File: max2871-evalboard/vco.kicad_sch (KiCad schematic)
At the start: 44 parts

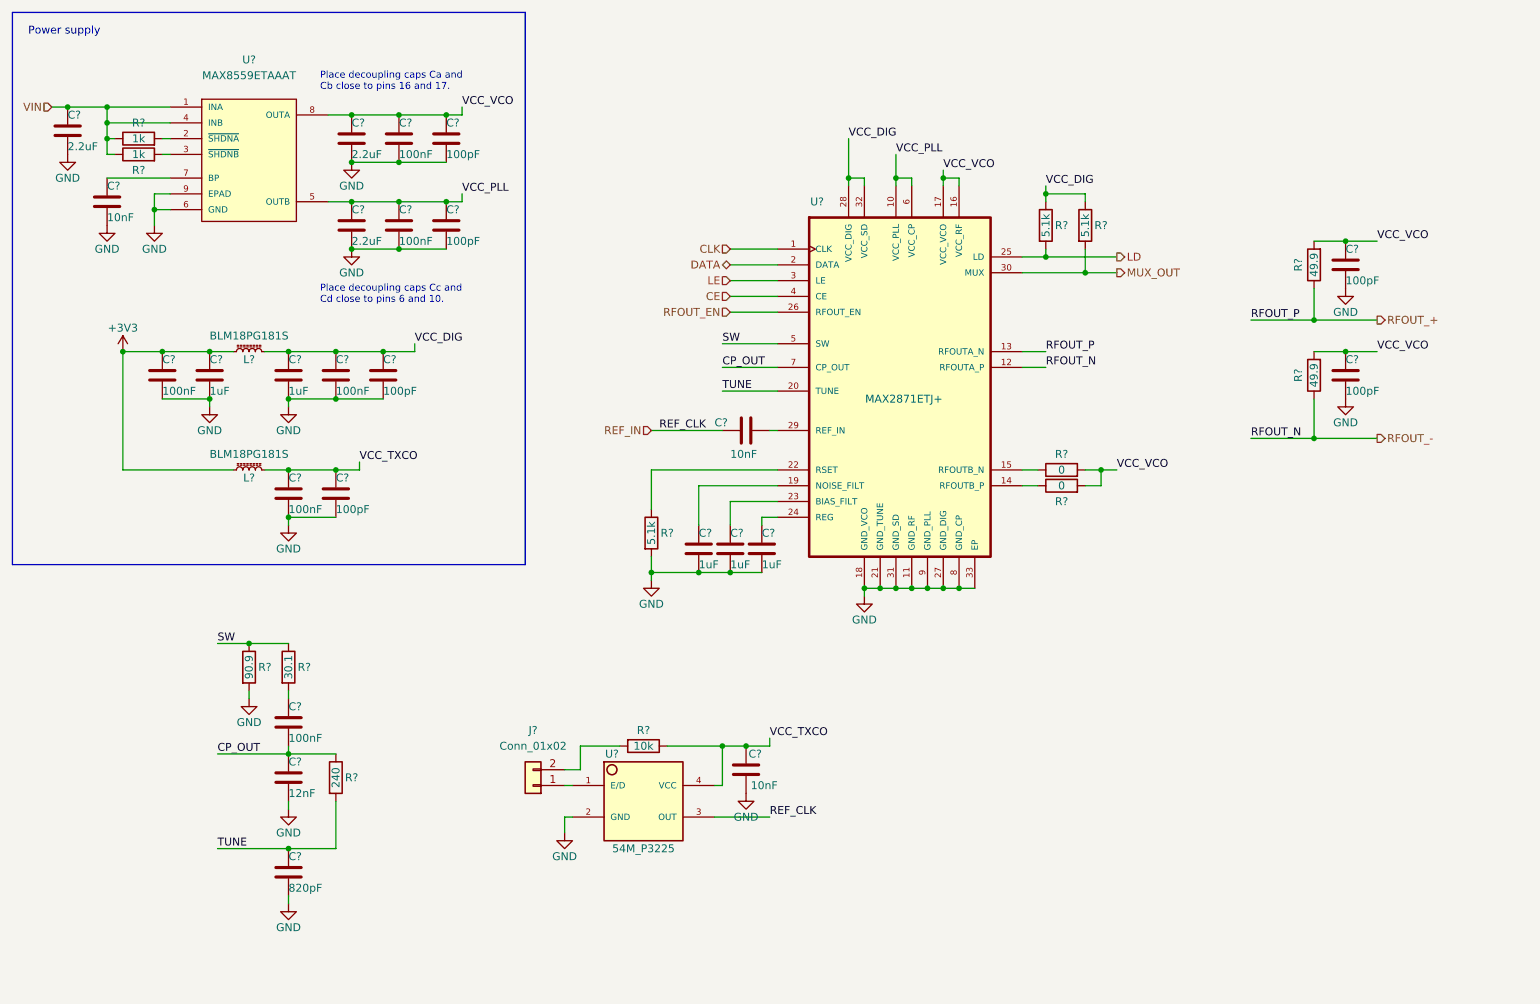
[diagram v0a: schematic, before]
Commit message: Finish schematic - create PCB
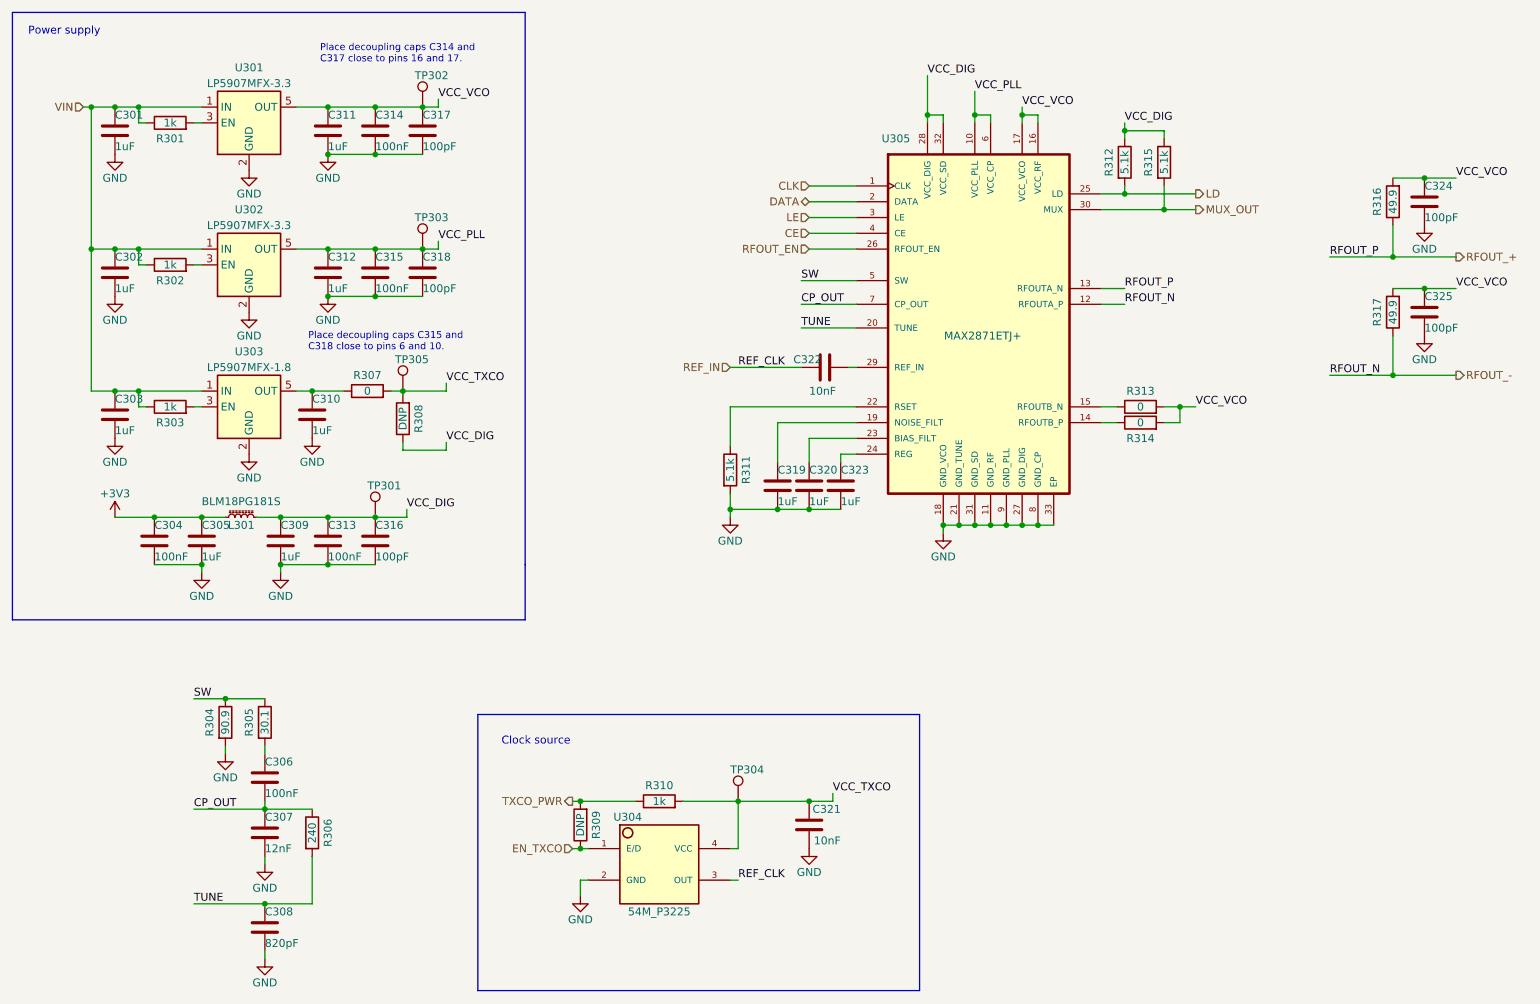
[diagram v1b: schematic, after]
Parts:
- removed C? (x3): 2.2uF, Capacitor_SMD:C_0603_1608Metric, symbol Device:C
- removed C?: 1uF, Capacitor_SMD:C_0402_1005Metric, symbol Device:C
- removed C?: 100pF, Capacitor_SMD:C_0402_1005Metric, symbol Device:C
- removed C?: 10nF, Capacitor_SMD:C_0402_1005Metric, symbol Device:C
- removed C?: 100nF, Capacitor_SMD:C_0402_1005Metric, symbol Device:C
- removed J?: Conn_01x02, Connector_PinHeader_2.54mm:PinHeader_2x01_P2.54mm_Horizontal, symbol Connector_Generic:Conn_01x02
- removed L?: BLM18PG181S, Inductor_SMD:L_0603_1608Metric, symbol Device:L_Ferrite_Small
- removed R?: 1k, Resistor_SMD:R_0402_1005Metric, symbol Device:R
- removed R?: 10k, Resistor_SMD:R_0402_1005Metric, symbol Device:R
- removed U?: MAX8559ETAAAT, MAX8559ETAAAT:SON65P300X300X80-9N, symbol MAX8559ETAAAT:MAX8559ETAAAT
- added C301, C302, C303, C309, C310, C311, C312: 1uF, Capacitor_SMD:C_0402_1005Metric, symbol Device:C
- added R301, R303, R310: 1k, Resistor_SMD:R_0402_1005Metric, symbol Device:R
- added R307: 0, Resistor_SMD:R_0402_1005Metric, symbol Device:R
- added R308, R309: DNP, Resistor_SMD:R_0402_1005Metric, symbol Device:R
- added TP301, TP302, TP303, TP304, TP305: (no value), TestPoint:TestPoint_Pad_D1.5mm, symbol Connector:TestPoint
- added U301, U302: LP5907MFX-3.3, Package_TO_SOT_SMD:SOT-23-5, symbol Regulator_Linear:LP5907MFX-3.3
- added U303: LP5907MFX-1.8, Package_TO_SOT_SMD:SOT-23-5, symbol Regulator_Linear:LP5907MFX-1.8
- C304, C306, C313, C314, C315: renamed from C?; Partnumber (none) -> CL05F104ZO5NNNC
- C305, C319, C320, C323: renamed from C?; LCSC (none) -> C126521; Manufacturer (none) -> Murata; Part Number (none) -> GCM155C71A105KE38D; Partnumber (none) -> GCM155C71A105KE38D
- C307: renamed from C?; LCSC (none) -> C113786; Manufacturer (none) -> YAGEO; Part Number (none) -> CC0402KRX7R8BB123; Partnumber (none) -> CC0402KRX7R8BB123
- C308: renamed from C?; LCSC (none) -> C107031; Manufacturer (none) -> YAGEO; Part Number (none) -> CC0402KRX7R9BB821; Partnumber (none) -> CC0402KRX7R9BB821
- C316, C317, C318, C324, C325: renamed from C?; Partnumber (none) -> CC0402KRX7R7BB101
- C321, C322: renamed from C?; Partnumber (none) -> TMK105B7103KVHF
- L301: renamed from L?; Partnumber (none) -> BLM18PG181SH1D
- R302: renamed from R?; LCSC (none) -> C705665; Manufacturer (none) -> YAGEO; Part Number (none) -> RT0402CRE071KL; Partnumber (none) -> RT0402CRE071KL
- R304: renamed from R?; LCSC (none) -> C852950; Manufacturer (none) -> YAGEO; Part Number (none) -> RT0402BRD0790R9L; Partnumber (none) -> RT0402BRD0790R9L
- R305, R306, R316, R317: renamed from R?; Partnumber (none) -> PTFR0402B49R9N9
- R311, R312, R315: renamed from R?; LCSC (none) -> C351692; Manufacturer (none) -> Resistor Today; Part Number (none) -> PTFR0402B5K10N9; Partnumber (none) -> PTFR0402B5K10N9
- R313, R314: renamed from R?; Partnumber (none) -> PA0402-R-070RL
- U304: renamed from U?; Partnumber (none) -> O3254000153350
- gave numbers to parts that had none: 1
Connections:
- net GND: now also C301.2, C302.2, C303.2, C309.2, C310.2, C311.2, C312.2, U301.2 (GND), U302.2 (GND), U303.2 (GND)
- net VCC_DIG: now also C309.1, R308.1, TP301.1
- net VCC_PLL: now also C312.1, TP303.1, U302.5 (OUT)
- net VCC_TXCO: now also R307.2, R308.2, R310.2, TP304.1, TP305.1
- net VCC_VCO: now also C311.1, TP302.1, U301.5 (OUT)
- net VIN: now also C301.1, C302.1, C303.1, R301.1, R303.1, U301.1 (IN), U302.1 (IN), U303.1 (IN)
- net EN_TXCO: now reaches U304.1 (E/D)
- net EN_TXCO: now also R309.1
- net at R302.2: now also U302.3 (EN)
- new net: C310.1, R307.1, U303.5 (OUT)
- new net: R303.2, U303.3 (EN)
- new net: R301.2, U301.3 (EN)
- new net TXCO_PWR: R309.2, R310.1
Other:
- note added: "Clock source"
- note added: "Place decoupling caps C314 and C317 close to pins 16 and 17."
- note added: "Place decoupling caps C315 and C318 close to pins 6 and 10."
- note removed: "Place decoupling caps Ca and Cb close to pins 16 and 17."
- note removed: "Place decoupling caps Cc and Cd close to pins 6 and 10."
- moved on the sheet: C304, C305, C306, C307, C308, C313, C314, C315, C316, C317, C318, C319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
